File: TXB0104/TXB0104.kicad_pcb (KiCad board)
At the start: 2 copper layers, 13 x 15.5 mm, 8 parts, among them J1 Conn_01x06, J2 Conn_01x06

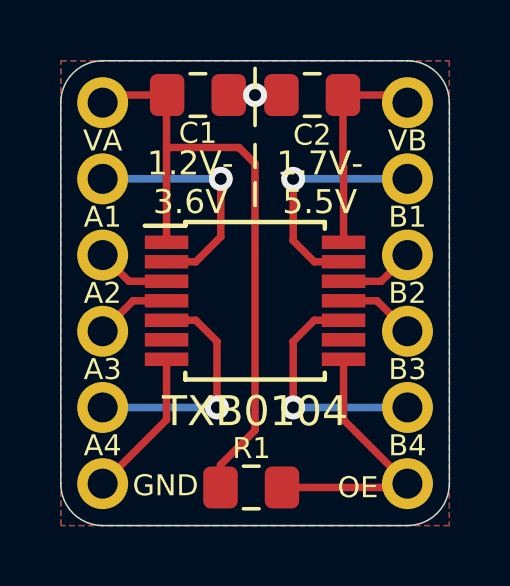
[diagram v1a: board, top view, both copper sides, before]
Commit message: Silkscreen Updated
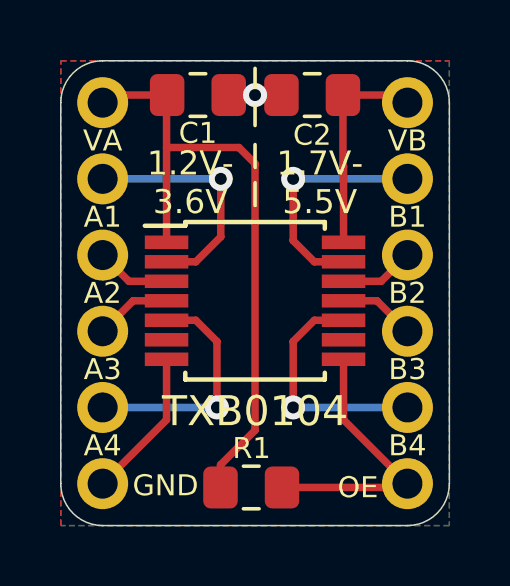
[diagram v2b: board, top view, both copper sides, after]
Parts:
- R1: value R_US -> 10k
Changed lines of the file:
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@@
   (general
     (thickness 1.6)
-    (drawings 29)
-    (tracks 50)
+    (drawings 33)
+    (tracks 51)
     (zones 0)
     (modules 8)
@@
   (layers
     (0 F.Cu signal)
-    (31 B.Cu signal hide)
+    (31 B.Cu signal)
     (32 B.Adhes user hide)
     (33 F.Adhes user hide)
@@
       (effects (font (size 0.7 0.7) (thickness 0.13)))
     )
-    (fp_text value R_US (at 0 1.65) (layer F.Fab)
+    (fp_text value 10k (at 0 1.65) (layer F.Fab)
       (effects (font (size 1 1) (thickness 0.15)))
     )
@@
     )
   )
+  (dimension 12.7 (width 0.15) (layer F.SilkS)
+    (gr_text "12.700 mm" (at 126.649 104.902 270) (layer F.SilkS)
+      (effects (font (size 1 1) (thickness 0.15)) hide)
+    )
+    (feature1 (pts (xy 122.174 111.252) (xy 125.935421 111.252)))
+    (feature2 (pts (xy 122.174 98.552) (xy 125.935421 98.552)))
+    (crossbar (pts (xy 125.349 98.552) (xy 125.349 111.252)))
+    (arrow1a (pts (xy 125.349 111.252) (xy 124.762579 110.125496)))
+    (arrow1b (pts (xy 125.349 111.252) (xy 125.935421 110.125496)))
+    (arrow2a (pts (xy 125.349 98.552) (xy 124.762579 99.678504)))
+    (arrow2b (pts (xy 125.349 98.552) (xy 125.935421 99.678504)))
+  )
+  (dimension 15.494 (width 0.15) (layer F.SilkS)
+    (gr_text "15.494 mm" (at 129.443 104.902 270) (layer F.SilkS)
+      (effects (font (size 1 1) (thickness 0.15)) hide)
+    )
+    (feature1 (pts (xy 123.571 112.649) (xy 128.729421 112.649)))
+    (feature2 (pts (xy 123.571 97.155) (xy 128.729421 97.155)))
+    (crossbar (pts (xy 128.143 97.155) (xy 128.143 112.649)))
+    (arrow1a (pts (xy 128.143 112.649) (xy 127.556579 111.522496)))
+    (arrow1b (pts (xy 128.143 112.649) (xy 128.729421 111.522496)))
+    (arrow2a (pts (xy 128.143 97.155) (xy 127.556579 98.281504)))
+    (arrow2b (pts (xy 128.143 97.155) (xy 128.729421 98.281504)))
+  )
+  (dimension 10.16 (width 0.15) (layer F.SilkS)
+    (gr_text "10.160 mm" (at 117.094 94.331) (layer F.SilkS)
+      (effects (font (size 1 1) (thickness 0.15)) hide)
+    )
+    (feature1 (pts (xy 122.174 98.552) (xy 122.174 95.044579)))
+    (feature2 (pts (xy 112.014 98.552) (xy 112.014 95.044579)))
+    (crossbar (pts (xy 112.014 95.631) (xy 122.174 95.631)))
+    (arrow1a (pts (xy 122.174 95.631) (xy 121.047496 96.217421)))
+    (arrow1b (pts (xy 122.174 95.631) (xy 121.047496 95.044579)))
+    (arrow2a (pts (xy 112.014 95.631) (xy 113.140504 96.217421)))
+    (arrow2b (pts (xy 112.014 95.631) (xy 113.140504 95.044579)))
+  )
+  (dimension 12.954 (width 0.15) (layer F.SilkS)
+    (gr_text "12.954 mm" (at 117.094 91.791) (layer F.SilkS)
+      (effects (font (size 1 1) (thickness 0.15)) hide)
+    )
+    (feature1 (pts (xy 123.571 97.155) (xy 123.571 92.504579)))
+    (feature2 (pts (xy 110.617 97.155) (xy 110.617 92.504579)))
+    (crossbar (pts (xy 110.617 93.091) (xy 123.571 93.091)))
+    (arrow1a (pts (xy 123.571 93.091) (xy 122.444496 93.677421)))
+    (arrow1b (pts (xy 123.571 93.091) (xy 122.444496 92.504579)))
+    (arrow2a (pts (xy 110.617 93.091) (xy 111.743504 93.677421)))
+    (arrow2b (pts (xy 110.617 93.091) (xy 111.743504 92.504579)))
+  )
   (gr_text "1.7V-\n5.5V" (at 119.253 101.219) (layer F.SilkS)
     (effects (font (size 0.8 0.8) (thickness 0.13)))
@@
   (segment (start 120.044 105.806) (end 119.069 105.806) (width 0.25) (layer F.Cu) (net 8))
   (segment (start 119.069 105.806) (end 118.364 106.511) (width 0.25) (layer F.Cu) (net 8))
-  (segment (start 118.364 108.712) (end 122.174 108.712) (width 0.25) (layer B.Cu) (net 8))
+  (segment (start 118.364 108.712) (end 118.872 108.712) (width 0.25) (layer B.Cu) (net 8))
+  (segment (start 118.872 108.712) (end 122.174 108.712) (width 0.25) (layer B.Cu) (net 8))
   (segment (start 121.158 105.156) (end 122.174 106.172) (width 0.25) (layer F.Cu) (net 9))
   (segment (start 120.044 105.156) (end 121.158 105.156) (width 0.25) (layer F.Cu) (net 9))
